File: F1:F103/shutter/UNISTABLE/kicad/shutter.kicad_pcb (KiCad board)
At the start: 2 copper layers, 61 x 42.5 mm, 49 parts, among them J1 ccd, J10 shutter, J11 USB_B, J2 hall, J3 ShtrPower, J4 SWD, J5 5Vext, J6 5v, J7 GND, J8 3v3, J9 USART1, Q1 IRL3303, Q2 DTA114Y, U1 LM1117-3.3, U2 STM32F103C6Tx, U3 USBLC6-2SC6, Y1 NX5032GA-8MHz

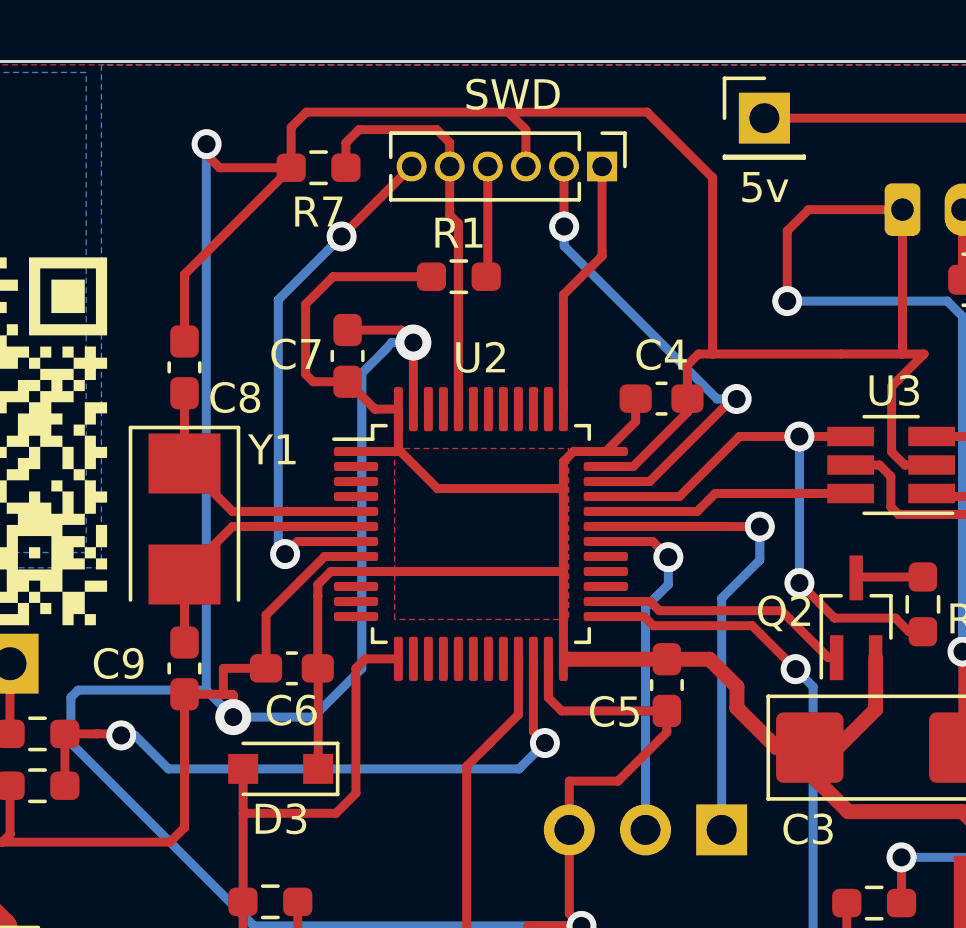
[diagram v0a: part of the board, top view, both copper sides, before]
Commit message: Unistable shutter
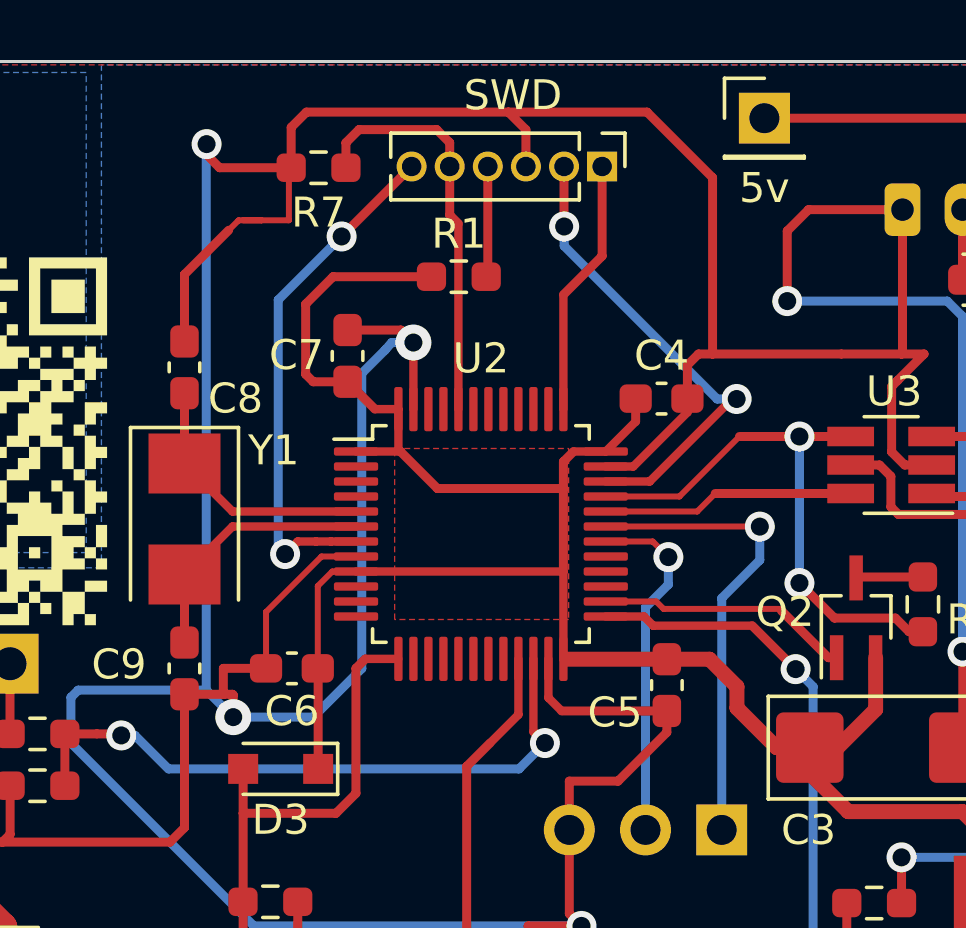
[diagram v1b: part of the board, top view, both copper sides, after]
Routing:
- net GND: track 285.1 -> 286.8 mm
